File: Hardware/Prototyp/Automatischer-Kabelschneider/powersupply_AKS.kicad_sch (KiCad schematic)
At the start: 4 parts, among them J1 USB_C_Receptacle_USB2.0_16P, U1 AP63203WU, U3 CYPD3177-24LQ

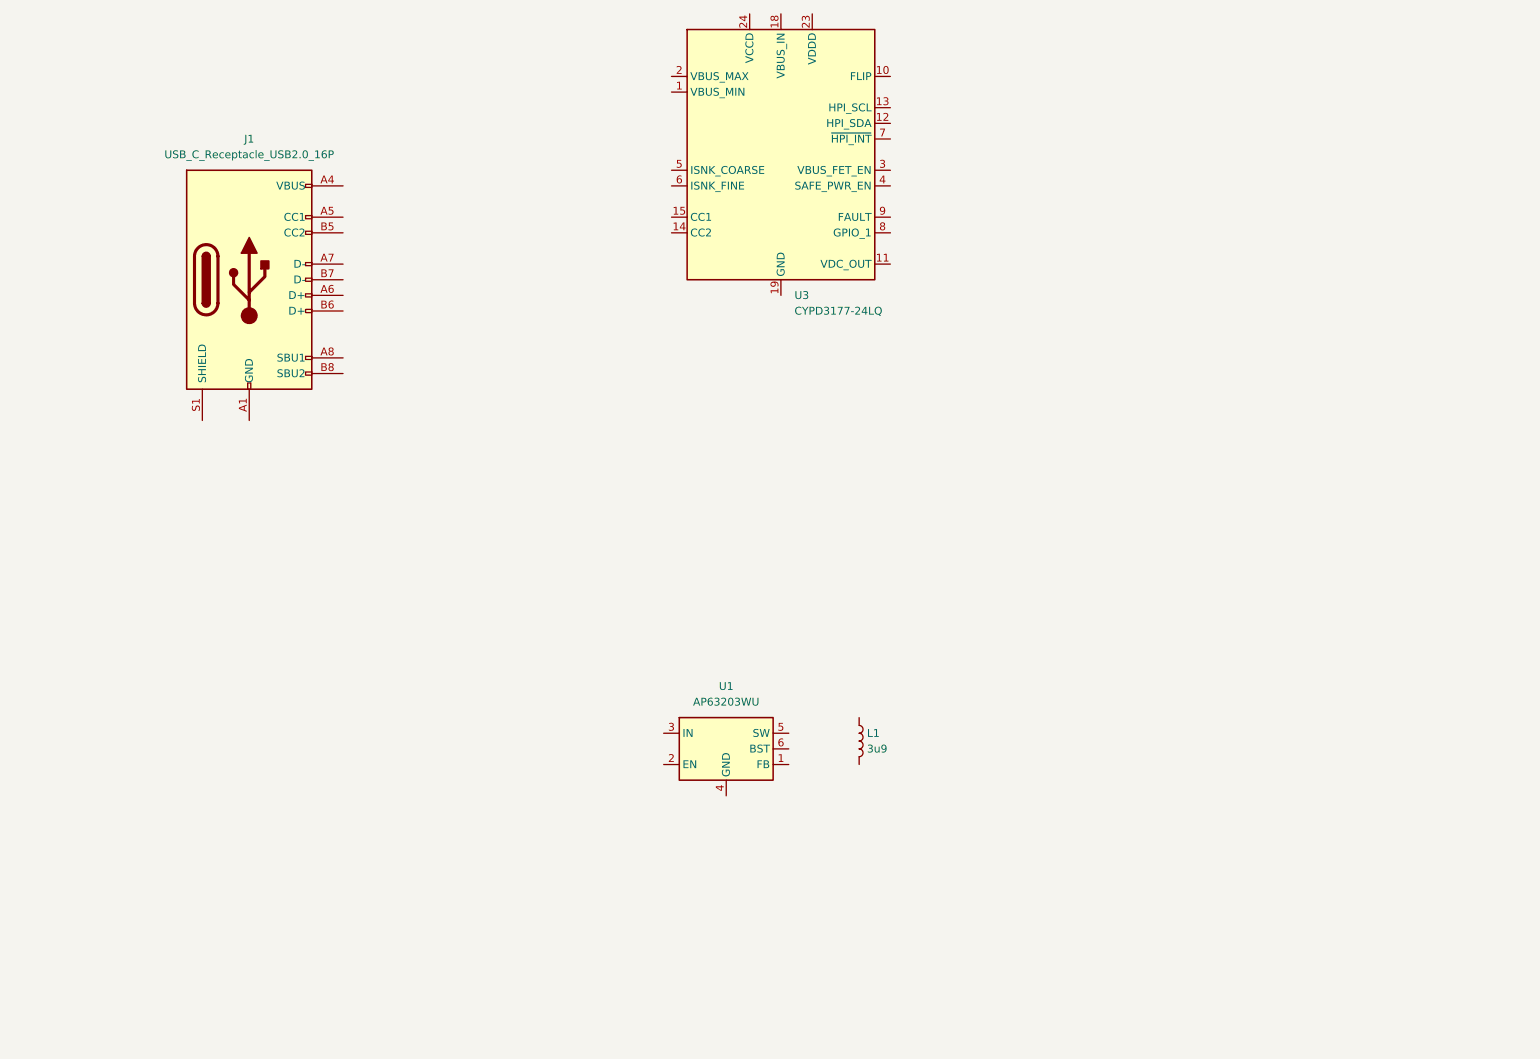
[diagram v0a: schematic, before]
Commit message: 20240410
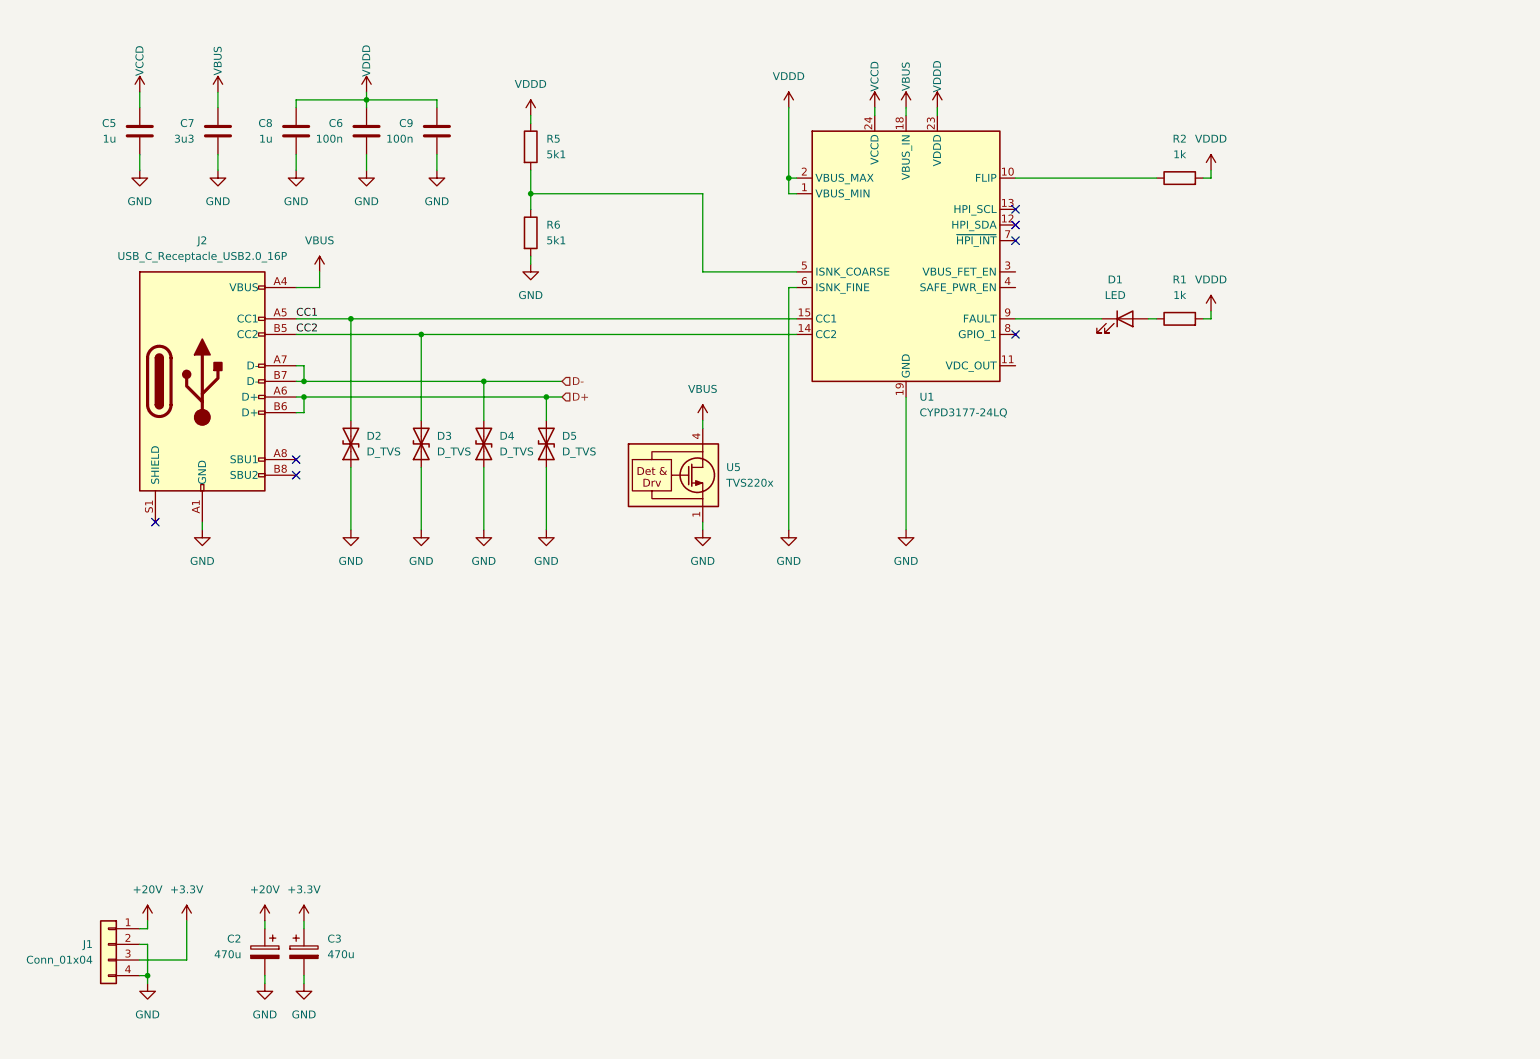
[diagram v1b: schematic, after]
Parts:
- removed J1: USB_C_Receptacle_USB2.0_16P, Connector_USB:USB_C_Receptacle_GCT_USB4105-xx-A_16P_TopMnt_Horizontal, symbol Connector:USB_C_Receptacle_USB2.0_16P
- removed L1: 3u9, Inductor_SMD:L_Wuerth_MAPI-4020, symbol Device:L
- removed U1: AP63203WU, Package_TO_SOT_SMD:TSOT-23-6, symbol Regulator_Switching:AP63203WU
- removed U3: CYPD3177-24LQ, Package_DFN_QFN:QFN-24-1EP_4x4mm_P0.5mm_EP2.75x2.75mm, symbol Interface_USB:CYPD3177-24LQ
- added C2, C3: 470u, Capacitor_SMD:C_Elec_8x10.2, symbol Device:C_Polarized
- added C5, C8: 1u, Capacitor_SMD:C_0805_2012Metric, symbol Device:C
- added C6, C9: 100n, Capacitor_SMD:C_0805_2012Metric, symbol Device:C
- added C7: 3u3, Capacitor_SMD:C_0805_2012Metric, symbol Device:C
- added D1: LED, Diode_SMD:D_0805_2012Metric, symbol Device:LED
- added D2, D3, D4, D5: D_TVS, Diode_SMD:D_0603_1608Metric, symbol Device:D_TVS
- added J1: Conn_01x04, Connector_Phoenix_GMSTB:PhoenixContact_GMSTBA_2,5_4-G-7,62_1x04_P7.62mm_Horizontal, symbol Connector_Generic:Conn_01x04
- added J2: USB_C_Receptacle_USB2.0_16P, Connector_USB:USB_C_Receptacle_GCT_USB4105-xx-A_16P_TopMnt_Horizontal, symbol Connector:USB_C_Receptacle_USB2.0_16P
- added R1, R2: 1k, Resistor_SMD:R_0805_2012Metric, symbol Device:R
- added R5, R6: 5k1, Resistor_SMD:R_0805_2012Metric, symbol Device:R
- added U1: CYPD3177-24LQ, Package_DFN_QFN:QFN-24-1EP_4x4mm_P0.5mm_EP2.75x2.75mm, symbol Interface_USB:CYPD3177-24LQ
- added U5: TVS220x, Package_SON:WSON-6-1EP_2x2mm_P0.65mm_EP1x1.6mm, symbol Power_Protection:TVS2200DRV
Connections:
- new net: R2.1, U1.10 (FLIP)
- new net: R5.2, R6.1, U1.5 (ISNK_COARSE)
- new net: D1.1 (K), U1.9 (FAULT)
- new net: D1.2 (A), R1.1
- new net +20V: C2.1, J1.1 (Pin_1)
- new net +3.3V: C3.1, J1.3 (Pin_3)
- new net CC1: D2.2 (A2), J2.A5 (CC1), U1.15 (CC1)
- new net CC2: D3.2 (A2), J2.B5 (CC2), U1.14 (CC2)
- new net D+: D5.2 (A2), J2.A6 (D+), J2.B6 (D+)
- new net D-: D4.2 (A2), J2.A7 (D-), J2.B7 (D-)
- new net GND: C2.2, C3.2, C5.2, C6.2, C7.2, C8.2, C9.2, D2.1 (A1), D3.1 (A1), D4.1 (A1), D5.1 (A1), J1.2 (Pin_2), J1.4 (Pin_4), J2.A1 (GND), J2.A12 (GND), J2.B1 (GND), J2.B12 (GND), R6.2, U1.19 (GND), U1.22 (GND), U1.25 (GND), U1.6 (ISNK_FINE), U5.1 (GND), U5.2 (GND), U5.3 (GND), U5.7 (GND)
- new net VBUS: C7.1, J2.A4 (VBUS), J2.A9 (VBUS), J2.B4 (VBUS), J2.B9 (VBUS), U1.18 (VBUS_IN), U5.4 (IN), U5.5 (IN), U5.6 (IN)
- new net VCCD: C5.1, U1.24 (VCCD)
- new net VDDD: C6.1, C8.1, C9.1, R1.2, R2.2, R5.1, U1.1 (VBUS_MIN), U1.2 (VBUS_MAX), U1.23 (VDDD)
- no-connect marks 0 -> 7

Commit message: 20240411
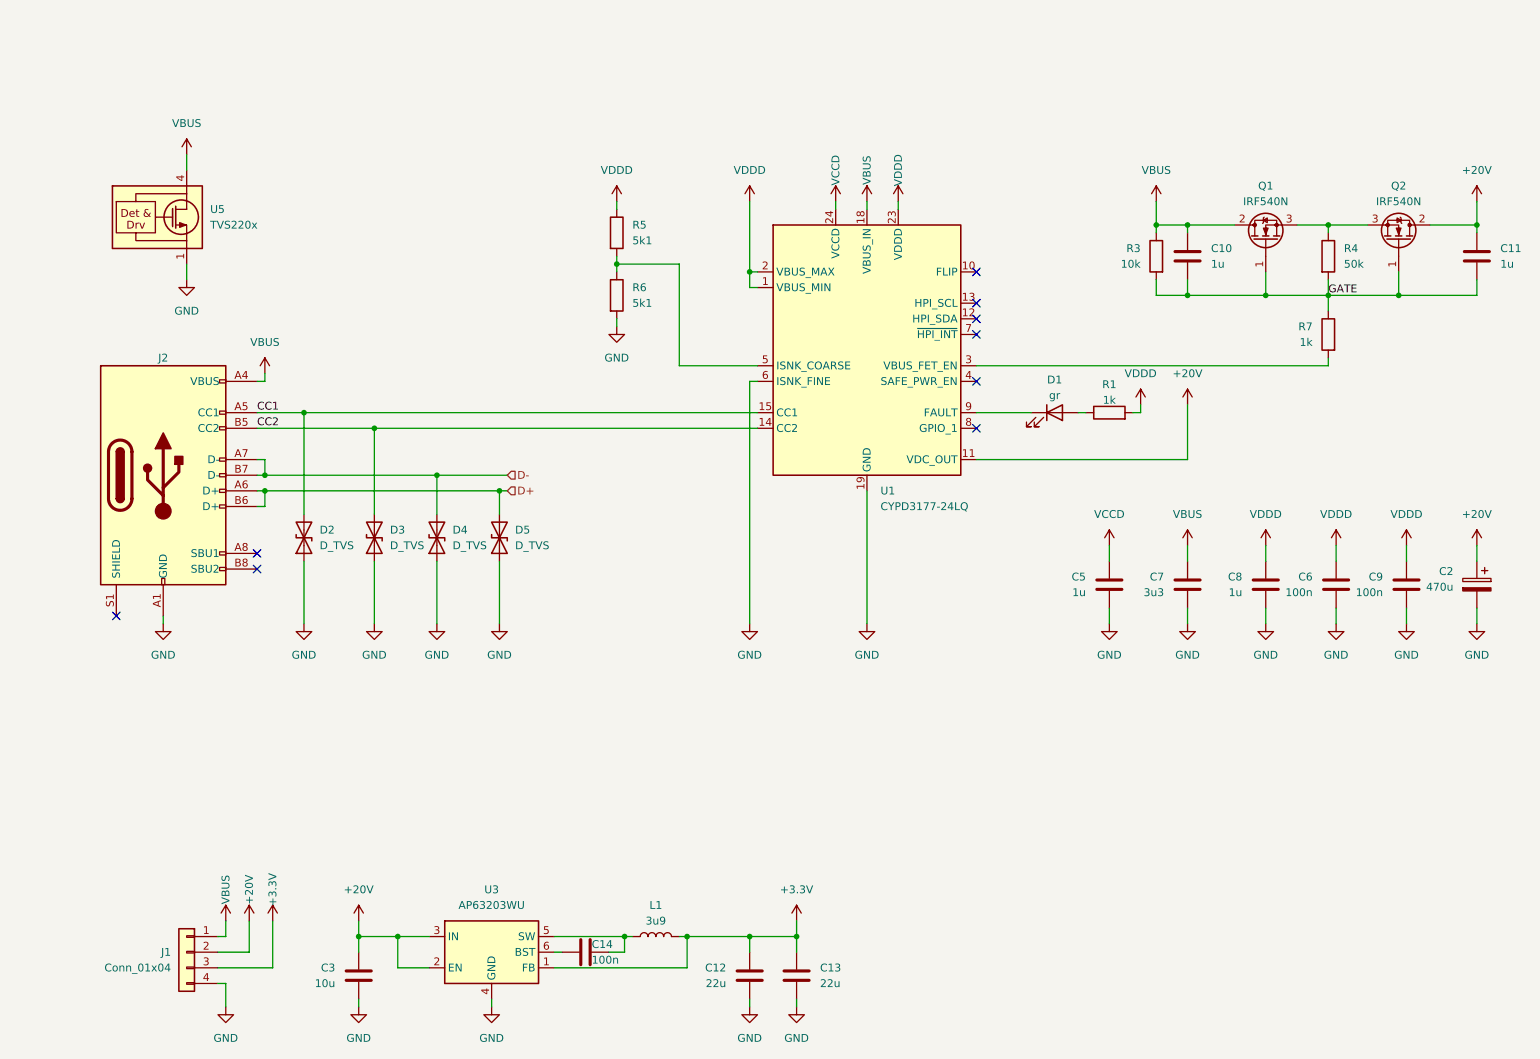
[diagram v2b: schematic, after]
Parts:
- removed C3: 470u, Capacitor_SMD:C_Elec_8x10.2, symbol Device:C_Polarized
- removed R2: 1k, Resistor_SMD:R_0805_2012Metric, symbol Device:R
- added C10, C11: 1u, Capacitor_SMD:C_0805_2012Metric, symbol Device:C
- added C12, C13: 22u, Capacitor_SMD:C_0805_2012Metric, symbol Device:C
- added C14: 100n, Capacitor_SMD:C_0805_2012Metric, symbol Device:C
- added C3: 10u, Capacitor_SMD:C_0805_2012Metric, symbol Device:C
- added L1: 3u9, Inductor_SMD_Wurth:L_Wurth_WE-LQSH-4020, symbol Device:L
- added Q1, Q2: IRF540N, Package_TO_SOT_THT:TO-220-3_Horizontal_TabDown, symbol Transistor_FET:IRF540N
- added R3: 10k, Resistor_SMD:R_0805_2012Metric, symbol Device:R
- added R4: 50k, Resistor_SMD:R_0805_2012Metric, symbol Device:R
- added R7: 1k, Resistor_SMD:R_0805_2012Metric, symbol Device:R
- added U3: AP63203WU, Package_TO_SOT_SMD:TSOT-23-6, symbol Regulator_Switching:AP63203WU
- D1: value LED -> gr
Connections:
- net +20V: now also J1.2 (Pin_2), U1.11 (VDC_OUT), C11.1, C3.1, Q2.2 (D), U3.2 (EN), U3.3 (IN); no longer J1.1 (Pin_1)
- net +3.3V: now also C12.1, C13.1, L1.2, U3.1 (FB)
- net GND: now also C12.2, C13.2, C3.2, U3.4 (GND); no longer J1.2 (Pin_2)
- net VBUS: now also J1.1 (Pin_1), C10.1, Q1.2 (D), R3.1
- net at U1.3 (VBUS_FET_EN): now also R7.2
- new net: C14.1, L1.1, U3.5 (SW)
- new net: C14.2, U3.6 (BST)
- new net: Q1.3 (S), Q2.3 (S), R4.1
- new net GATE: C10.2, C11.2, Q1.1 (G), Q2.1 (G), R3.2, R4.2, R7.1
- no-connect marks 7 -> 9
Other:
- moved on the sheet: C2, C5, C6, C7, C8, C9, D1, D2, D3, D4, D5, J1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
